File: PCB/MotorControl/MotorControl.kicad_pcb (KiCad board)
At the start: 2 copper layers, 45.5 x 34.5 mm, 11 parts, among them J1 Conn_01x05_Pin, J5 Conn_01x05_Pin, J6 USB_C_Receptacle_USB2.0_14P, J8 Conn_01x04_Socket, U1 PCA9685PW, U3 TC1262-33, U4 STM32L031K6Tx

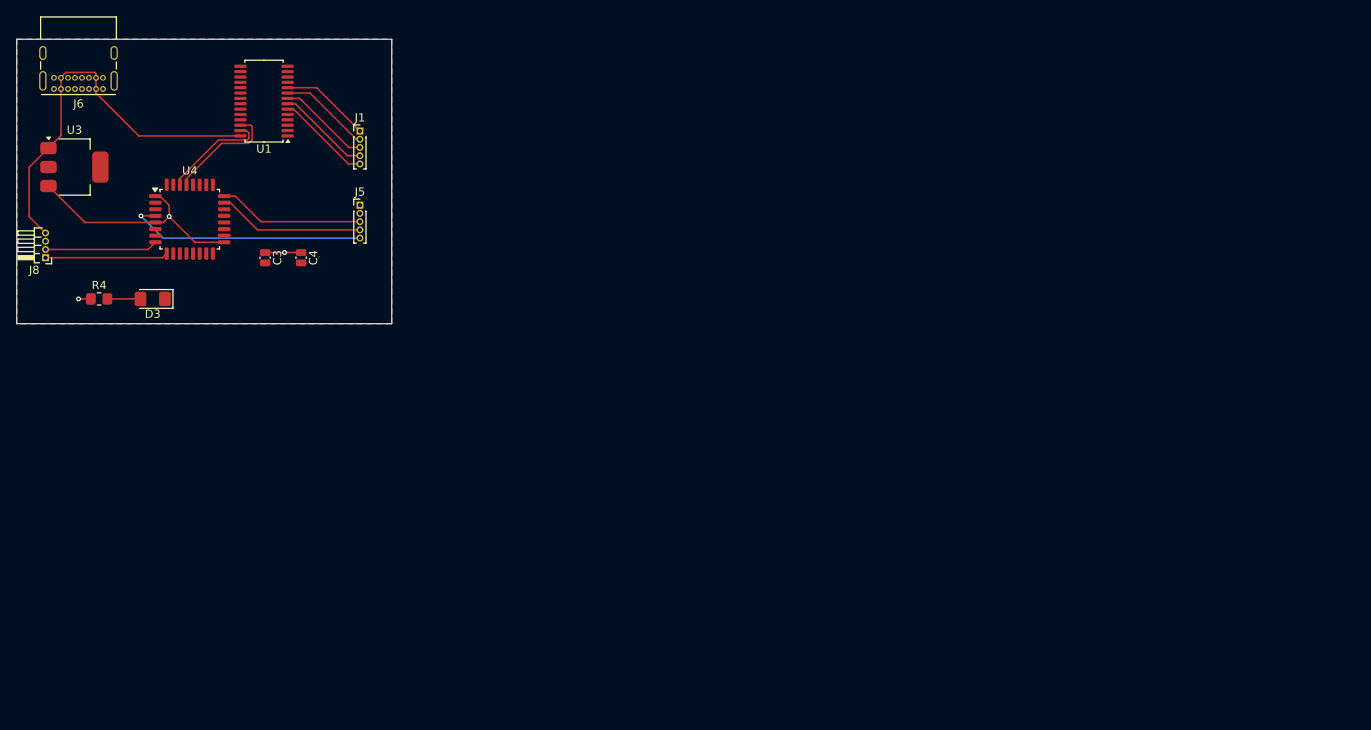
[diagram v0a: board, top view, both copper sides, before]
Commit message: Pushing
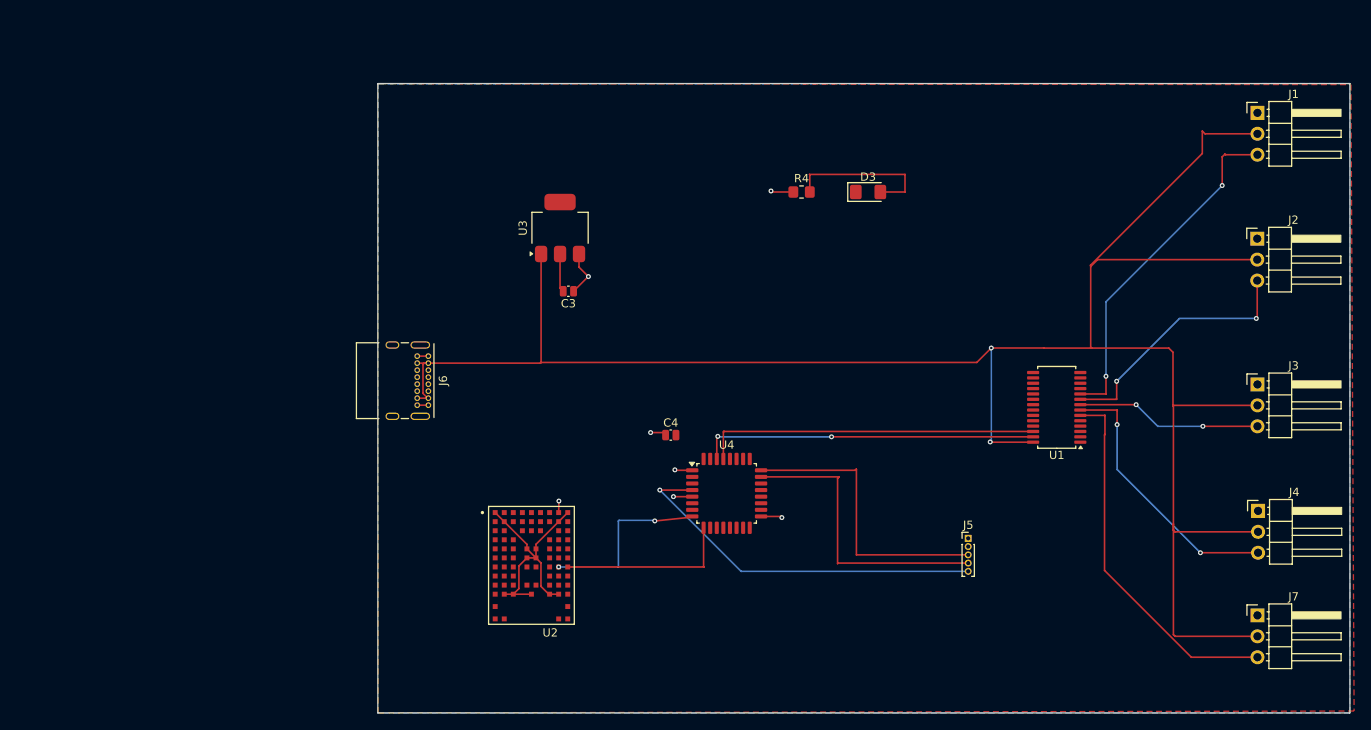
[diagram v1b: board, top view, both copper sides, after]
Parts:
- removed J8: Conn_01x04_Socket, Connector_PinHeader_1.00mm:PinHeader_1x04_P1.00mm_Horizontal
- added J2: Conn_01x03_Pin, Connector_PinHeader_2.54mm:PinHeader_1x03_P2.54mm_Horizontal, F.Cu at (185.0, 56.7)
- added J3: Conn_01x03_Pin, Connector_PinHeader_2.54mm:PinHeader_1x03_P2.54mm_Horizontal, F.Cu at (185.0, 74.4)
- added J4: Conn_01x03_Pin, Connector_PinHeader_2.54mm:PinHeader_1x03_P2.54mm_Horizontal, F.Cu at (185.1, 89.7)
- added J7: Conn_01x03_Pin, Connector_PinHeader_2.54mm:PinHeader_1x03_P2.54mm_Horizontal, F.Cu at (185.0, 102.4)
- added U2: NORA-W106-00B, NORA-W106-00B:XCVR_NORA-W106-00B, F.Cu at (96.9, 96.3)
- J1: value Conn_01x05_Pin -> Conn_01x03_Pin; footprint Connector_PinHeader_1.00mm:PinHeader_1x05_P1.00mm_Vertical -> Connector_PinHeader_2.54mm:PinHeader_1x03_P2.54mm_Horizontal
- moved J1 108.9 mm to (185.0, 41.4)
- moved U1 103.1 mm to (160.7, 77.2)
- moved D3 87.7 mm to (137.8, 51.0), turned to 0 degrees
- moved R4 86.2 mm to (129.7, 51.0)
- moved J5 84.1 mm to (149.9, 93.0)
- moved U4 73.1 mm to (120.6, 87.6)
- moved U3 59.4 mm to (100.4, 55.4), turned to 90 degrees
- moved J6 51.1 mm to (84.4, 70.9), turned to -90 degrees
- moved C4 49.7 mm to (113.9, 80.5), turned to 0 degrees
- moved C3 37.0 mm to (101.4, 63.1), turned to 180 degrees
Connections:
- J1 pad 1: Net-(J1-Pin_1) -> GND
- J1 pad 2: Net-(J1-Pin_2) -> 5V
- U1 pad 10: Net-(J1-Pin_1) -> Net-(J1-Pin_3)
- U1 pad 6: Net-(J1-Pin_5) -> Net-(J7-Pin_3)
- U1 pad 7: Net-(J1-Pin_4) -> Net-(J4-Pin_3)
- U1 pad 8: Net-(J1-Pin_3) -> Net-(J3-Pin_3)
- U1 pad 9: Net-(J1-Pin_2) -> Net-(J2-Pin_3)
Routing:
- net 5V: track 47.9 -> 254.3 mm, vias 0 -> 2
- net Net-(J7-Pin_3): track 0.00 -> 44.7 mm
- net GND: track 0.00 -> 37.8 mm
- net Net-(J4-Pin_3): track 0.00 -> 33.2 mm, vias 0 -> 2
- net Net-(J2-Pin_3): track 0.00 -> 31.4 mm, vias 0 -> 2
- net Net-(J1-Pin_3): track 11.2 -> 42.3 mm, vias 0 -> 2
- net Net-(U1-SDA): track 12.9 -> 41.3 mm, vias 0 -> 2
- net Net-(U1-SCL): track 13.8 -> 40.9 mm
- net Net-(J3-Pin_3): track 0.00 -> 22.9 mm, vias 0 -> 2
- net SWDIO: track 17.8 -> 35.9 mm
- net SWSCLK: track 17.7 -> 35.6 mm
- net +3.3V: track 34.1 -> 17.5 mm, vias 3 -> 7
- net NRST: track 29.4 -> 45.4 mm
- net Net-(D3-A): track 4.01 -> 18.9 mm
- net Net-(J1-Pin_5): track 11.5 -> 0.00 mm
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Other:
- board size 45.5 x 34.5 mm -> 117.9 x 76.4 mm
